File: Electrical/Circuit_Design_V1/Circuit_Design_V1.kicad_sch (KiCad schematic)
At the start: 18 parts, among them Q1 NMOS, U1 STM32G474RETx

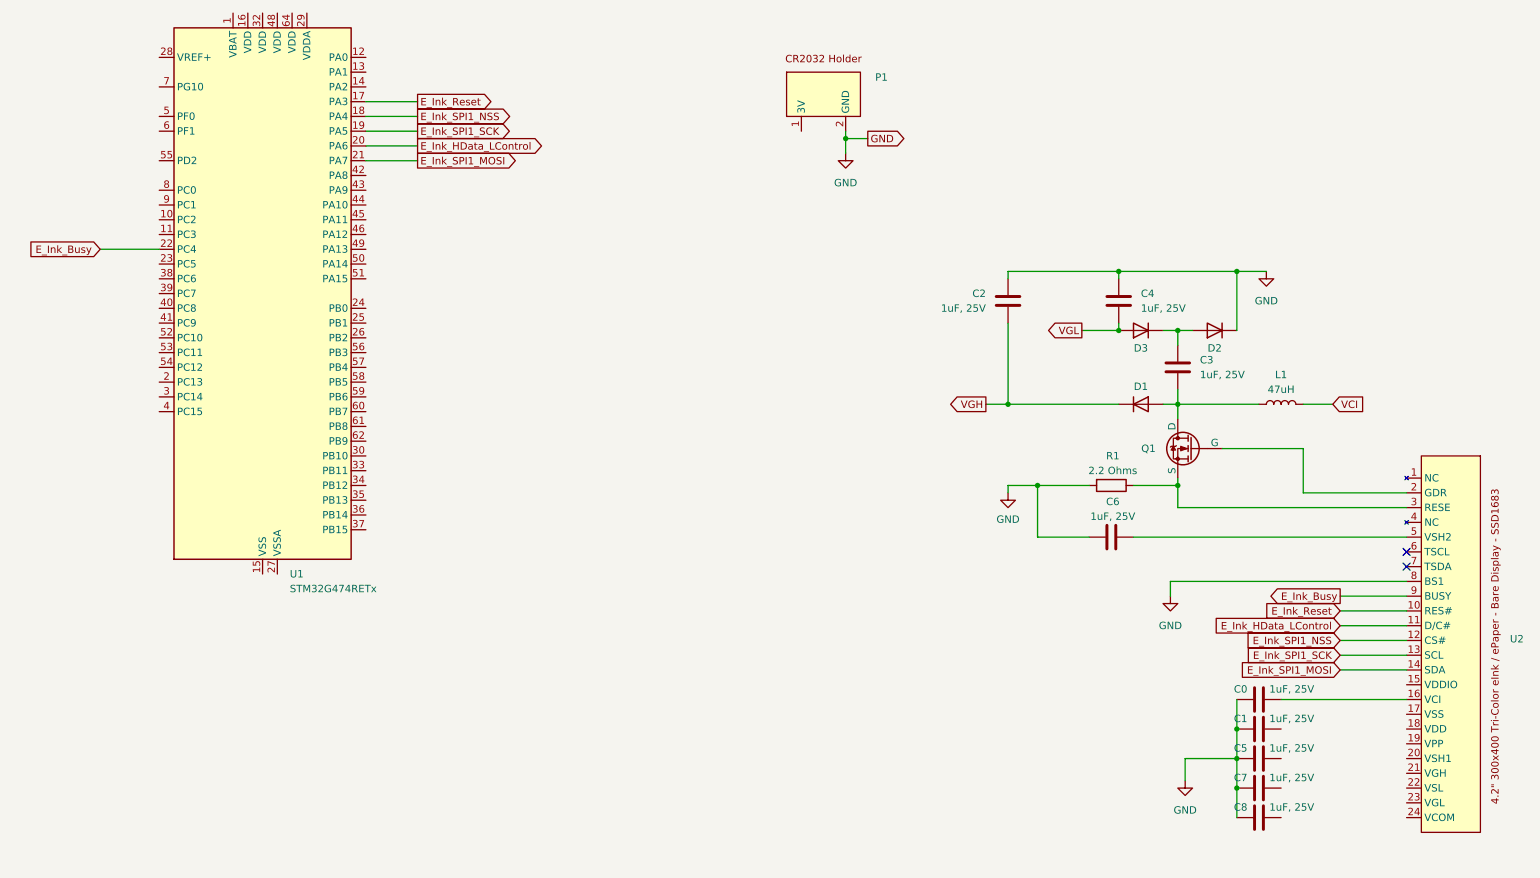
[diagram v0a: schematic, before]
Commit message: #3 Creating the system diagram.
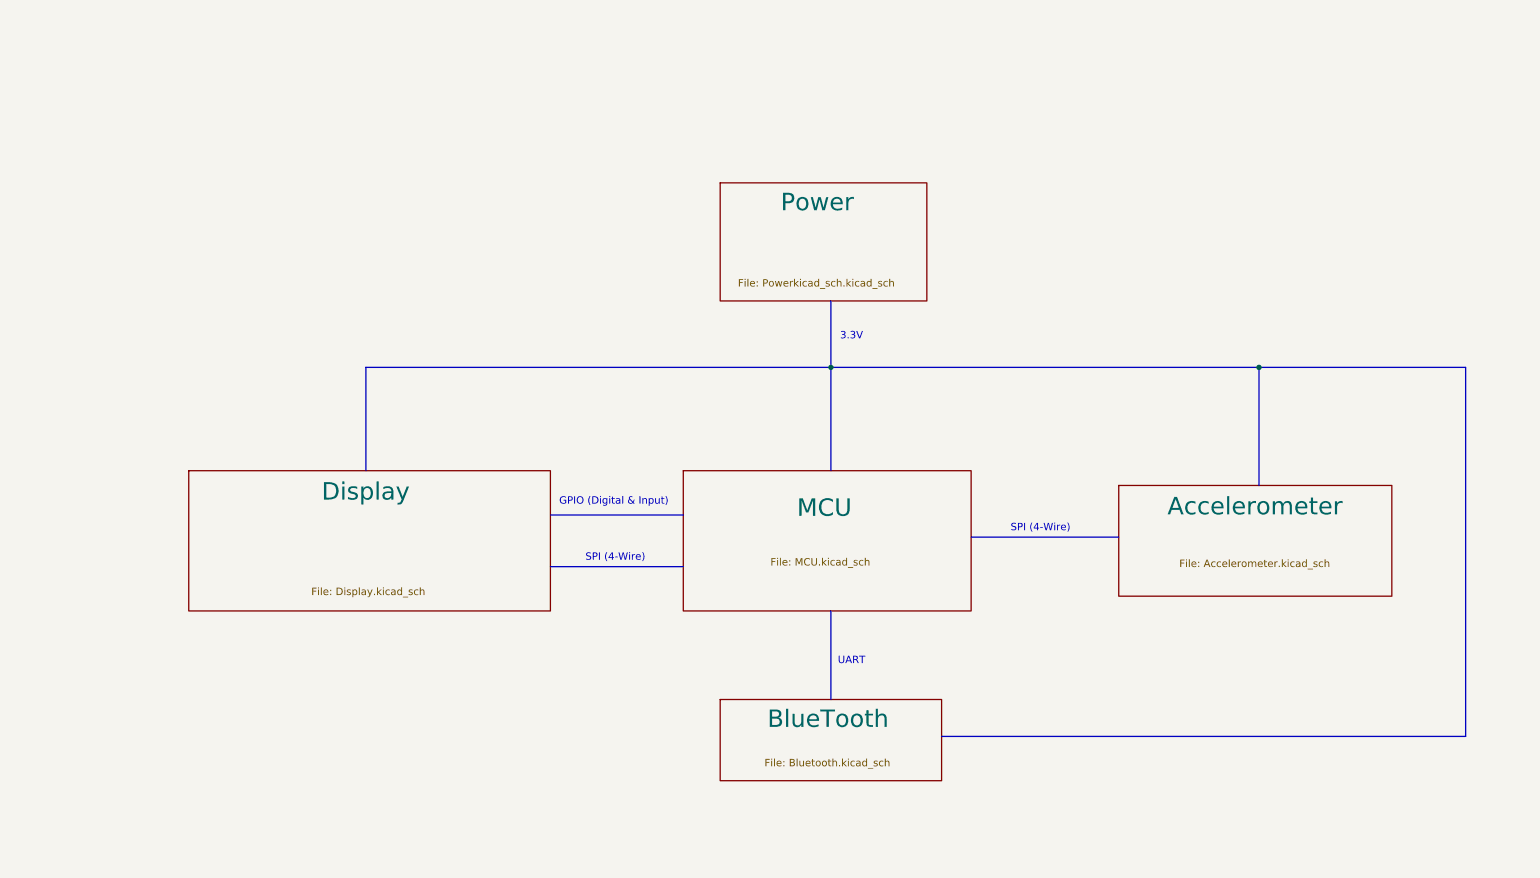
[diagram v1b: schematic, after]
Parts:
- removed C0, C1, C2, C3, C4, C5, C6, C7, C8: 1uF, 25V, symbol Device:C
- removed D1, D2, D3: D, symbol Device:D
- removed L1: 47uH, symbol Device:L
- removed P1: ~, symbol Etchasketch_hardware_symbol_library:20mm_Coin_Cell_Breakout_Board_(CR2032)
- removed Q1: NMOS, symbol Simulation_SPICE:NMOS
- removed R1: 2.2 Ohms, symbol Device:R
- removed U1: STM32G474RETx, Package_QFP:LQFP-64_10x10mm_P0.5mm, symbol MCU_ST_STM32G4:STM32G474RETx
- removed U2: ~, symbol Etchasketch_hardware_symbol_library:4.2{dblquote}_300x400_Tri-Color_eInk_/_ePap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
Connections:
- no-connect marks 2 -> 0
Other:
- added sheet Accelerometer (Accelerometer.kicad_sch)
- added sheet BlueTooth (Bluetooth.kicad_sch)
- added sheet Display (Display.kicad_sch)
- added sheet MCU (MCU.kicad_sch)
- added sheet Power (Powerkicad_sch.kicad_sch)
- note added: "3.3V"
- note added: "GPIO (Digital & Input)"
- note added: "SPI (4-Wire)"
- note added: "UART"
- company: (none) -> AdrianTheHacker
- title: (none) -> Etchasketch System Design
